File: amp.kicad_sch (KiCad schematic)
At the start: 14 parts, among them IC301 MAX98357AETE+T, IC302 MAX98357AETE+T, J301 L_SPKR, J302 R_SPKR

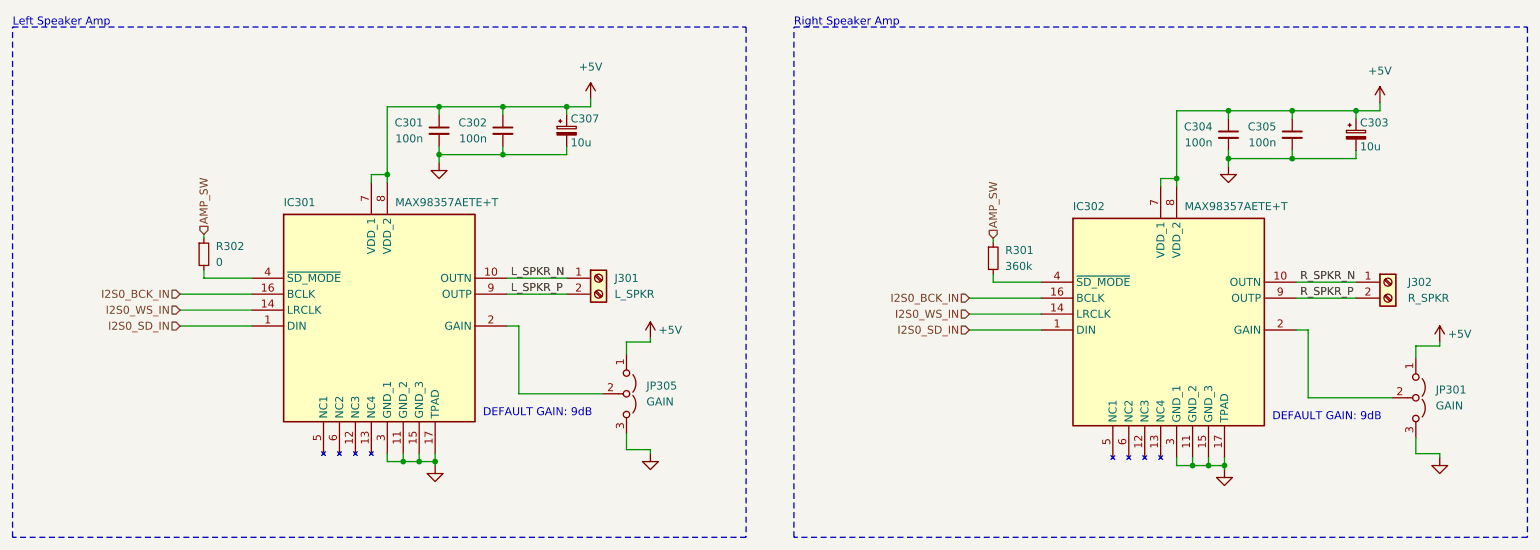
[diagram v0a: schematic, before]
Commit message: updated to rev 4
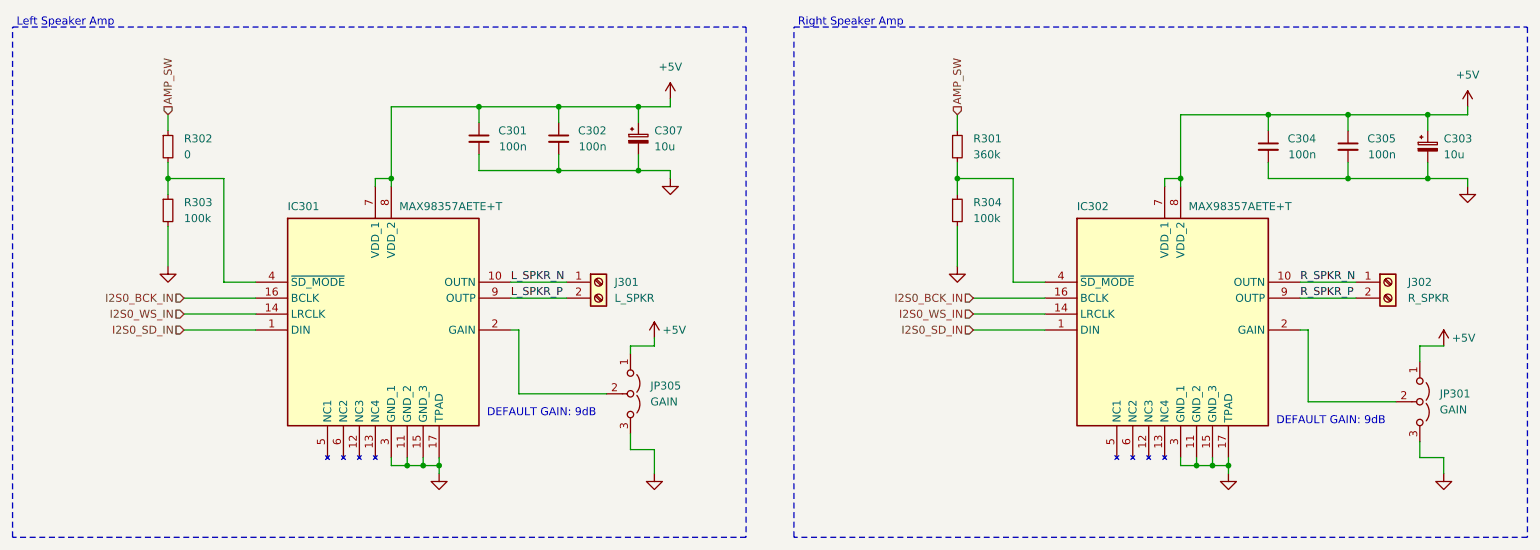
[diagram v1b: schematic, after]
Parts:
- added R303, R304: 100k, Resistor_SMD:R_0402_1005Metric, symbol Device:R_Small
- C301, C302, C304, C305: footprint Capacitor_SMD:C_0603_1608Metric -> Capacitor_SMD:C_0402_1005Metric; JLCPCB Part # (none) -> C1525; LCSC C1525 -> (none)
- C303, C307: footprint Capacitor_SMD:C_0805_2012Metric -> Capacitor_SMD:C_0603_1608Metric; JLCPCB Part # (none) -> C96446
- IC301, IC302: JLCPCB Part # (none) -> C910544; LCSC C910544 -> (none)
- R301: footprint Resistor_SMD:R_0603_1608Metric -> Resistor_SMD:R_0402_1005Metric; JLCPCB Part # (none) -> C45956; LCSC C45956 -> (none)
- R302: footprint Resistor_SMD:R_0603_1608Metric -> Resistor_SMD:R_0402_1005Metric; JLCPCB Part # (none) -> C17168; LCSC C45956 -> (none)
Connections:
- net GND: now also R303.2, R304.2
- net at IC301.4 (~{SD_MODE}), R302.2: now also R303.1
- net at IC302.4 (~{SD_MODE}), R301.2: now also R304.1
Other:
- moved on the sheet: C301, C302, C303, C304, C305, C307, IC301, IC302, J301, JP301, JP305, R302
